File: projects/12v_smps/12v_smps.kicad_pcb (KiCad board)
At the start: 6 copper layers, 7 parts, among them U2 TPSM82902SISR

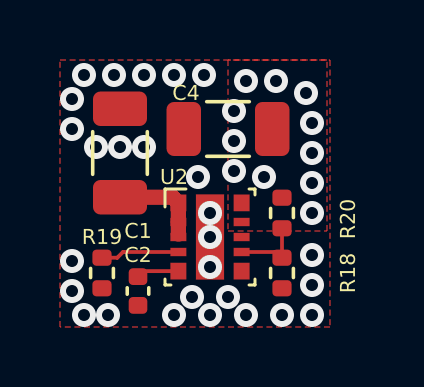
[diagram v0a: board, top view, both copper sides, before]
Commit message: wip
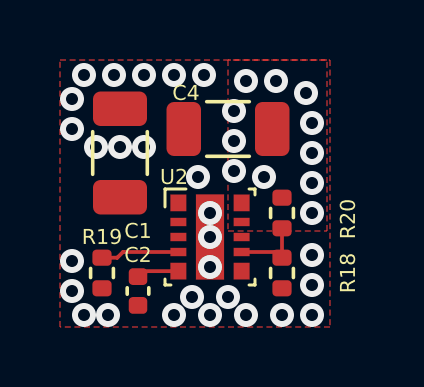
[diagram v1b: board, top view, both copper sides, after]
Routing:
- net /VIN: track 3.07 -> 0.00 mm
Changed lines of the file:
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@@
 		(property ki_fp_filters "R_*")
 		(sheetname "/")
+		(sheetfile "12v_smps.kicad_sch")
 		(attr smd)
 		(fp_line
@@
 		(property ki_fp_filters "uSIP11_SIS_TEX uSIP11_SIS_TEX-M uSIP11_SIS_TEX-L")
 		(sheetname "/")
+		(sheetfile "12v_smps.kicad_sch")
 		(attr smd)
 		(fp_line
@@
 		(property ki_fp_filters "R_*")
 		(sheetname "/")
+		(sheetfile "12v_smps.kicad_sch")
 		(attr smd dnp)
 		(fp_line
@@
 		(property ki_fp_filters "C_*")
 		(sheetname "/")
+		(sheetfile "12v_smps.kicad_sch")
 		(attr smd)
 		(fp_line
@@
 		(property ki_fp_filters "R_*")
 		(sheetname "/")
+		(sheetfile "12v_smps.kicad_sch")
 		(attr smd dnp)
 		(fp_line
@@
 		(property ki_fp_filters "C_*")
 		(sheetname "/")
+		(sheetfile "12v_smps.kicad_sch")
 		(attr smd dnp)
 		(fp_line
@@
 		(property ki_fp_filters "C_*")
 		(sheetname "/")
+		(sheetfile "12v_smps.kicad_sch")
 		(attr smd)
 		(fp_line
@@
 	)
 	(segment
-		(start 174.3459 60.262499)
-		(end 174.3459 60.899874)
-		(width 0.508)
-		(layer "F.Cu")
-		(net 3)
-	)
-	(segment
-		(start 174.3459 60.899874)
-		(end 174.3459 61.305426)
-		(width 0.508)
-		(layer "F.Cu")
-		(net 3)
-	)
-	(segment
-		(start 174.158401 60.075)
-		(end 174.3459 60.262499)
-		(width 0.508)
-		(layer "F.Cu")
-		(net 3)
-	)
-	(segment
-		(start 172.4 60.075)
-		(end 174.158401 60.075)
-		(width 0.508)
-		(layer "F.Cu")
-		(net 3)
-	)
-	(segment
